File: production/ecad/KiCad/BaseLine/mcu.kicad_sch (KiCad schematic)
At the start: 31 parts, among them J6 1332645, Q2 AO3400A, Q3 AO3400A, SW1 SW_Push, SW2 SW_Push, U4 ESP32-WROOM-32UE_M113EH6400UH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, U5 CP2102N-A02-GQFN28

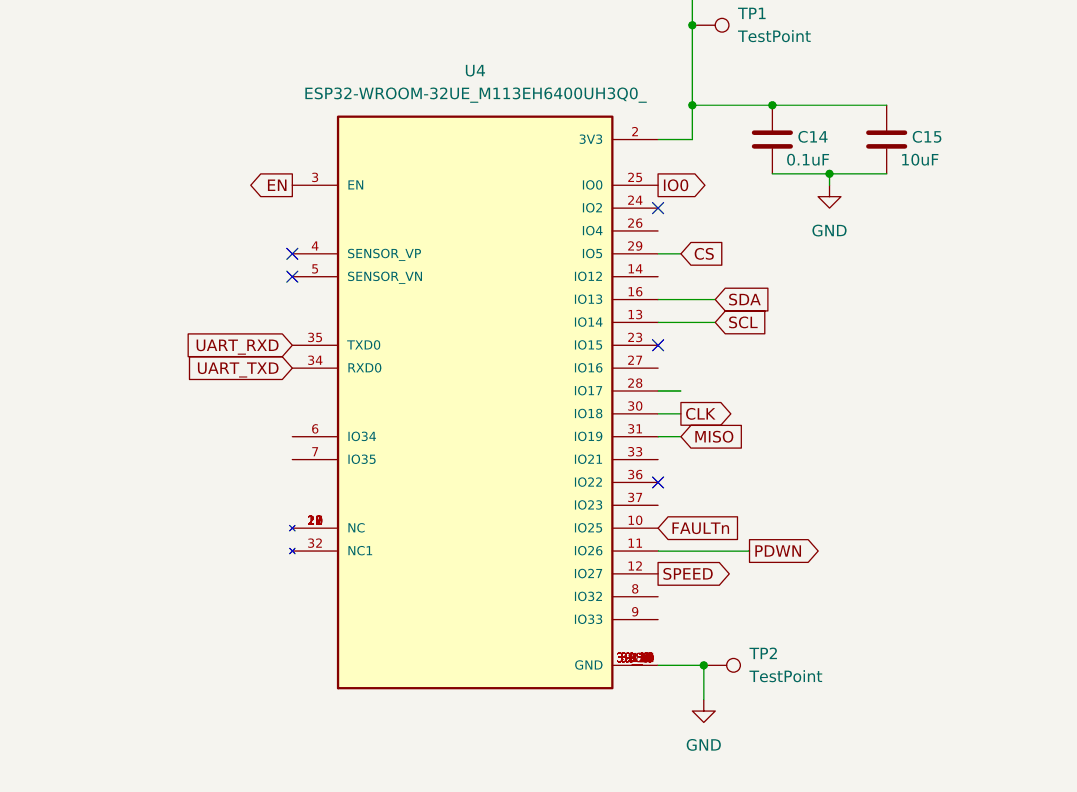
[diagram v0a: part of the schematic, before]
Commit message: Added 0 ohm resistors
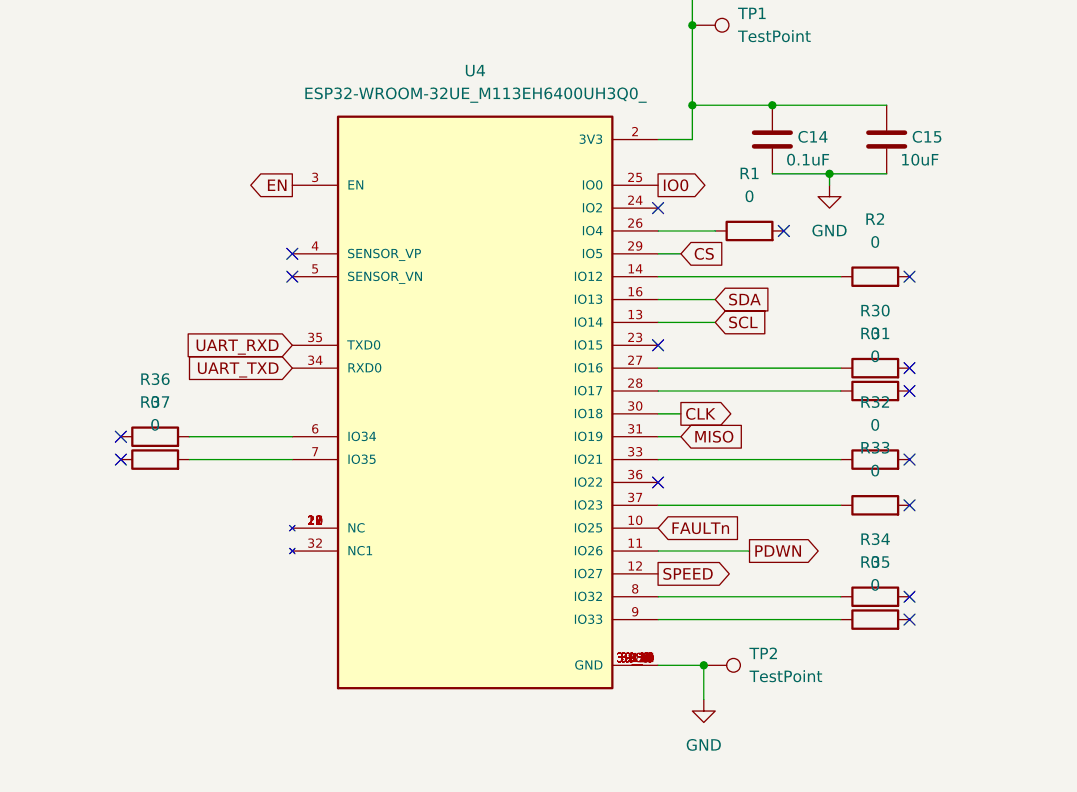
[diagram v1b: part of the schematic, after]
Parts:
- added R1, R2, R30, R31, R32, R33, R34, R35, R36, R37: 0, symbol Device:R
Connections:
- net at U4.14 (IO12): now also R2.1
- net at U4.26 (IO4): now also R1.1
- net at U4.27 (IO16): now also R30.1
- net at U4.28 (IO17): now also R31.1
- net at U4.33 (IO21): now also R32.1
- net at U4.37 (IO23): now also R33.1
- net at U4.6 (IO34): now also R36.2
- net at U4.7 (IO35): now also R37.2
- net at U4.8 (IO32): now also R34.1
- net at U4.9 (IO33): now also R35.1
- no-connect marks 19 -> 29
